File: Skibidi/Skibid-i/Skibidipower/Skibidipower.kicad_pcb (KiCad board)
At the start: 2 copper layers, 19 parts, among them J1 SparkOut, J2 Bat2, J3 Bat1, J5 Sparkout 48V, J6 Sparkin, Q1 SQM40P10-40L_GE3, Q2 SQ2318AES-T1_BE3

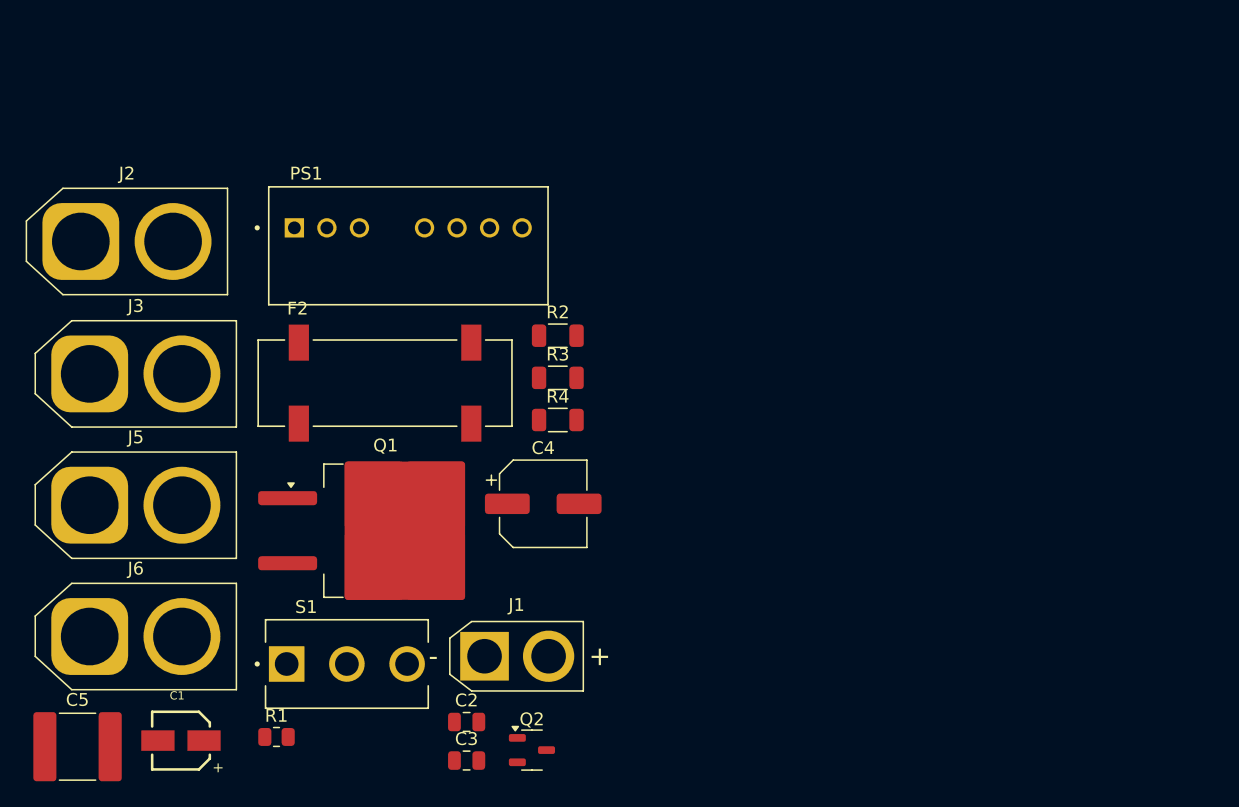
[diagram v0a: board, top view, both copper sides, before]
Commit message: skibidi rizz
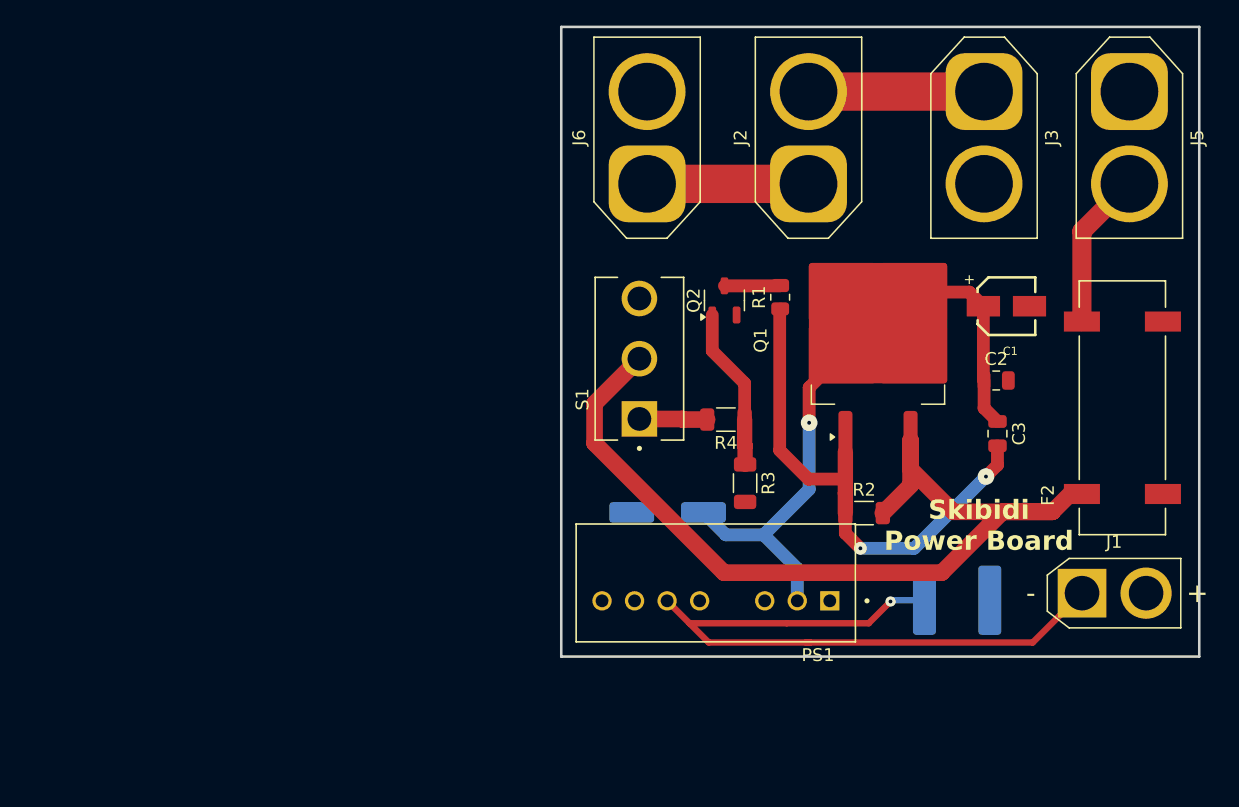
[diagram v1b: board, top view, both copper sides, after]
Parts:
- C4, C5: moved to B.Cu
- moved J5 87.3 mm to (218.1, 79.3), turned to -90 degrees
- moved J3 73.2 mm to (206.8, 79.3), turned to -90 degrees
- moved C1 72.8 mm to (208.5, 96.0), turned to 180 degrees
- moved C5 69.6 mm to (204.7, 119.0)
- moved F2 57.6 mm to (217.6, 104.0), turned to 90 degrees
- moved J2 57.0 mm to (193.1, 86.5), turned to 90 degrees
- moved J6 56.0 mm to (180.4, 86.5), turned to 90 degrees
- moved R1 52.2 mm to (190.8, 95.3), turned to 90 degrees
- moved C2 49.2 mm to (207.7, 101.8)
- moved C3 48.7 mm to (207.8, 106.0), turned to -90 degrees
- moved J1 46.9 mm to (214.4, 118.5)
- moved Q1 41.1 mm to (198.5, 98.9), turned to 90 degrees
- moved Q2 38.2 mm to (186.5, 95.6), turned to 90 degrees
- moved PS1 35.6 mm to (185.8, 117.7), turned to 180 degrees
- moved S1 33.0 mm to (179.8, 100.2), turned to 90 degrees
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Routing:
- net Net-(Q1-S): track 0.00 -> 73.2 mm
- net +12V: track 0.00 -> 57.0 mm, vias 0 -> 1
- net +48V: track 0.00 -> 43.7 mm, vias 0 -> 1
- net Net-(Q1-G): track 0.00 -> 41.7 mm, vias 0 -> 2
- net Net-(J2-Pin_2): track 0.00 -> 13.7 mm
- net Net-(Q2-G): track 0.00 -> 12.8 mm
- net Net-(J2-Pin_1): track 0.00 -> 12.6 mm
- net Net-(J5-Pin_2): track 0.00 -> 12.3 mm
- net Net-(R4-Pad2): track 0.00 -> 5.31 mm
- net Net-(Q2-D): track 0.00 -> 4.36 mm
- added copper zone on B.Cu, net GND
- added copper zone on F.Cu, net GND
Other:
- board outline added: 49.8 x 49.2 mm
- board text added: "Skibidi Power Board"
